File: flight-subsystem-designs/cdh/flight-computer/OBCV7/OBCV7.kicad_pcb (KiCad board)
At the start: 4 copper layers, 90.3 x 95.9 mm, 47 parts, among them U1 BEAGLEBONEBLACK, U3 TCAN337G, U4 MCP7940N-xSN, U5 ADM3485EARZ, U6 MAX706RESA+T, U7 TMP36xS

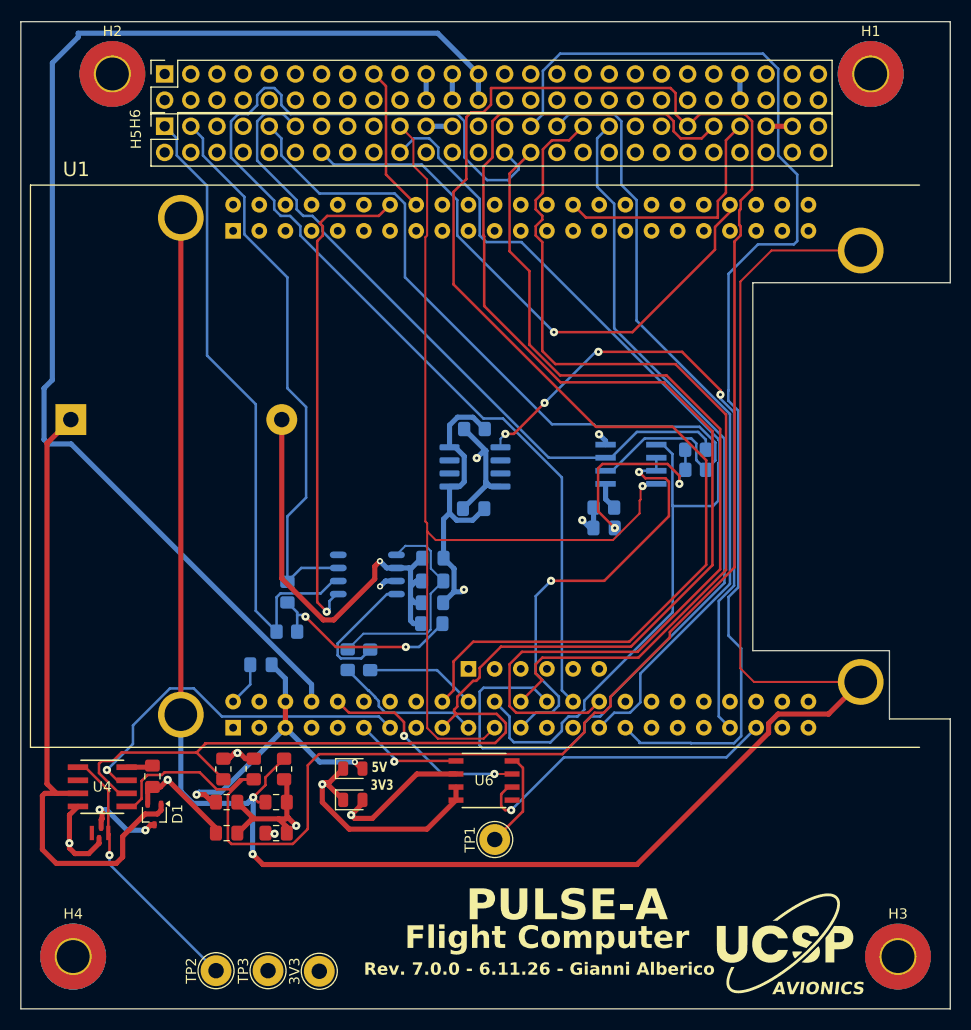
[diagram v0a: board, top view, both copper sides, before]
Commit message: New Footprint Fixes and Routing Improvements
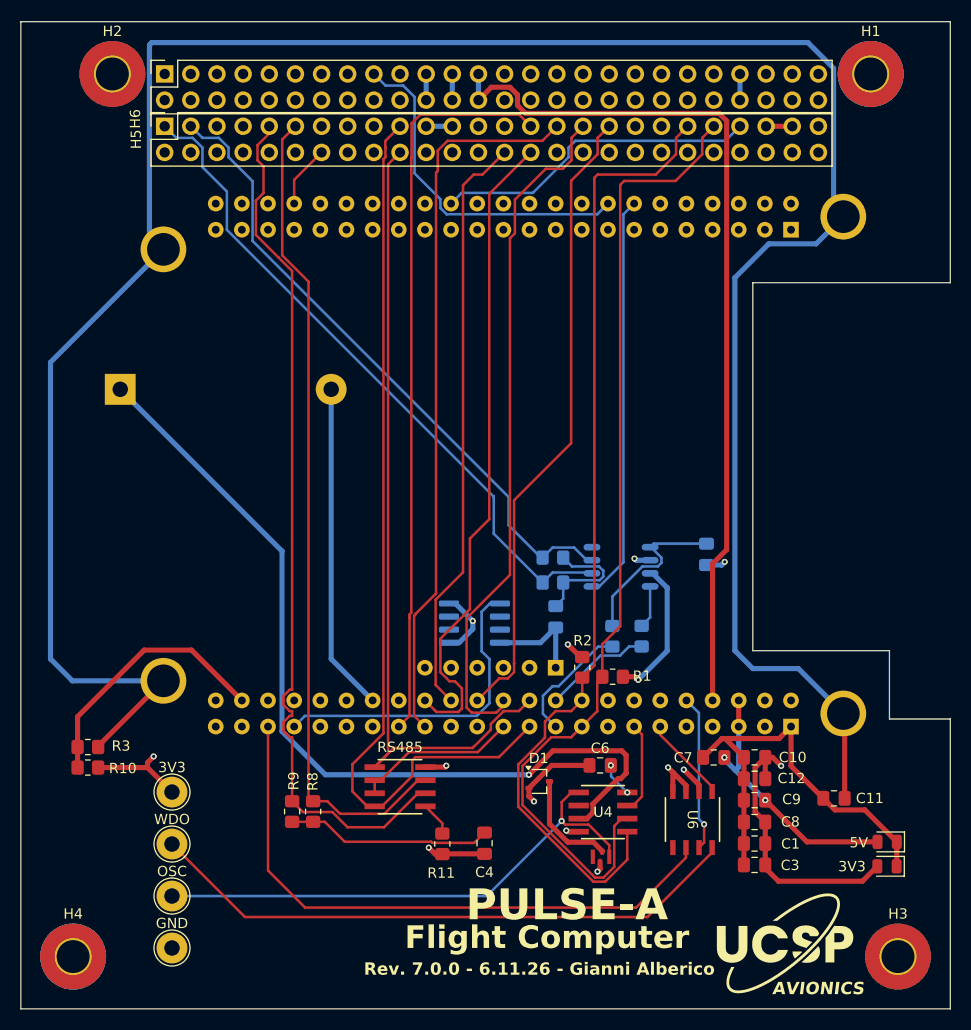
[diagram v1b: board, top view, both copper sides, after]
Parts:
- removed the 3V3 at (121.7, 122.6)
- removed D2: 5V, LED_SMD:LED_0805_2012Metric
- removed D3: 3V3, LED_SMD:LED_0805_2012Metric
- removed TP1: WDO, TestPoint:TestPoint_THTPad_D3.0mm_Drill1.5mm
- removed TP2: CLKOUT, TestPoint:TestPoint_THTPad_D3.0mm_Drill1.5mm
- removed TP3: GND, TestPoint:TestPoint_THTPad_D3.0mm_Drill1.5mm
- removed U5: ADM3485EARZ, Footprints:R_8_ADI
- removed U7: TMP36xS, Package_SO:SOIC-8_3.9x4.9mm_P1.27mm
- added 3V3: TestPoint, TestPoint:TestPoint_THTPad_D3.0mm_Drill1.5mm, F.Cu at (107.4, 105.2)
- added 3V3: 3V3, LED_SMD:LED_0805_2012Metric, F.Cu at (176.8, 112.4)
- added 5V: 5V, LED_SMD:LED_0805_2012Metric, F.Cu at (176.8, 110.1)
- added GND: GND, TestPoint:TestPoint_THTPad_D3.0mm_Drill1.5mm, F.Cu at (107.4, 120.4)
- added OSC: CLKOUT, TestPoint:TestPoint_THTPad_D3.0mm_Drill1.5mm, F.Cu at (107.4, 115.3)
- added RS485: ADM3485EARZ, Footprints:R_8_ADI, F.Cu at (129.5, 104.7)
- added TMP36XS: TMP36xS, Package_SO:SOIC-8_3.9x4.9mm_P1.27mm, B.Cu at (136.7, 88.8)
- added WDO: WDO, TestPoint:TestPoint_THTPad_D3.0mm_Drill1.5mm, F.Cu at (107.4, 110.3)
- C1, C10, C3, C4, C9, R10, R11, R8, R9: moved to F.Cu
- U1: moved to B.Cu
- moved C11 54.2 mm to (171.7, 105.8), turned to 180 degrees
- moved R9 51.4 mm to (119.0, 107.1), turned to -90 degrees
- moved C8 51.3 mm to (163.9, 108.1), turned to 180 degrees
- moved R8 51.1 mm to (121.1, 107.1), turned to 90 degrees
- moved R10 49.9 mm to (99.2, 102.8)
- moved C9 49.7 mm to (164.0, 106.0)
- moved XTAL1 48.7 mm to (148.9, 111.4)
- moved U4 48.7 mm to (149.2, 107.2)
- moved C7 47.5 mm to (160.0, 101.9), turned to 180 degrees
- moved C12 46.8 mm to (164.0, 103.9), turned to 180 degrees
- moved C6 43.5 mm to (148.9, 102.6), turned to 0 degrees
- moved C1 41.8 mm to (163.9, 110.2)
- moved C3 40.3 mm to (163.9, 112.3)
- moved R1 38.9 mm to (150.2, 94.0), turned to 0 degrees
- moved D1 37.5 mm to (143.0, 104.2), turned to 0 degrees
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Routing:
- net /I2C_SDA: track 257.7 -> 94.3 mm
- net /I2C_SCL: track 171.8 -> 95.5 mm
- net /SPI_CSO: track 110.6 -> 57.1 mm
- net /PPS: track 55.8 -> 6.07 mm, vias 1 -> 0
- net Net-(U6-*WDO): track 9.43 -> 58.5 mm
- net /SPI_SCLK: track 114.0 -> 71.5 mm
- net SYS_5V: track 121.4 -> 86.0 mm
- net Net-(C11-Pad1): track 205.5 -> 238.6 mm, vias 2 -> 0
- net /UART2_RX: track 94.0 -> 61.6 mm
- net /SPI_D1: track 93.7 -> 63.0 mm
- net /Temp: track 61.7 -> 31.2 mm, vias 4 -> 0
- net /GPIO3_20: track 30.8 -> 59.1 mm, vias 1 -> 0
- net /RTCC_MFP: track 35.7 -> 8.90 mm, vias 1 -> 0
- net /GPIO1_17: track 41.9 -> 15.9 mm, vias 2 -> 0
- net Net-(U4-X1): track 25.8 -> 51.5 mm
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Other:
- board text removed: "3V3"
- board text removed: "5V"
